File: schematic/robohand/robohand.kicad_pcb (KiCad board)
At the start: 2 copper layers, 1 part, among them U1 ESP32-CAM

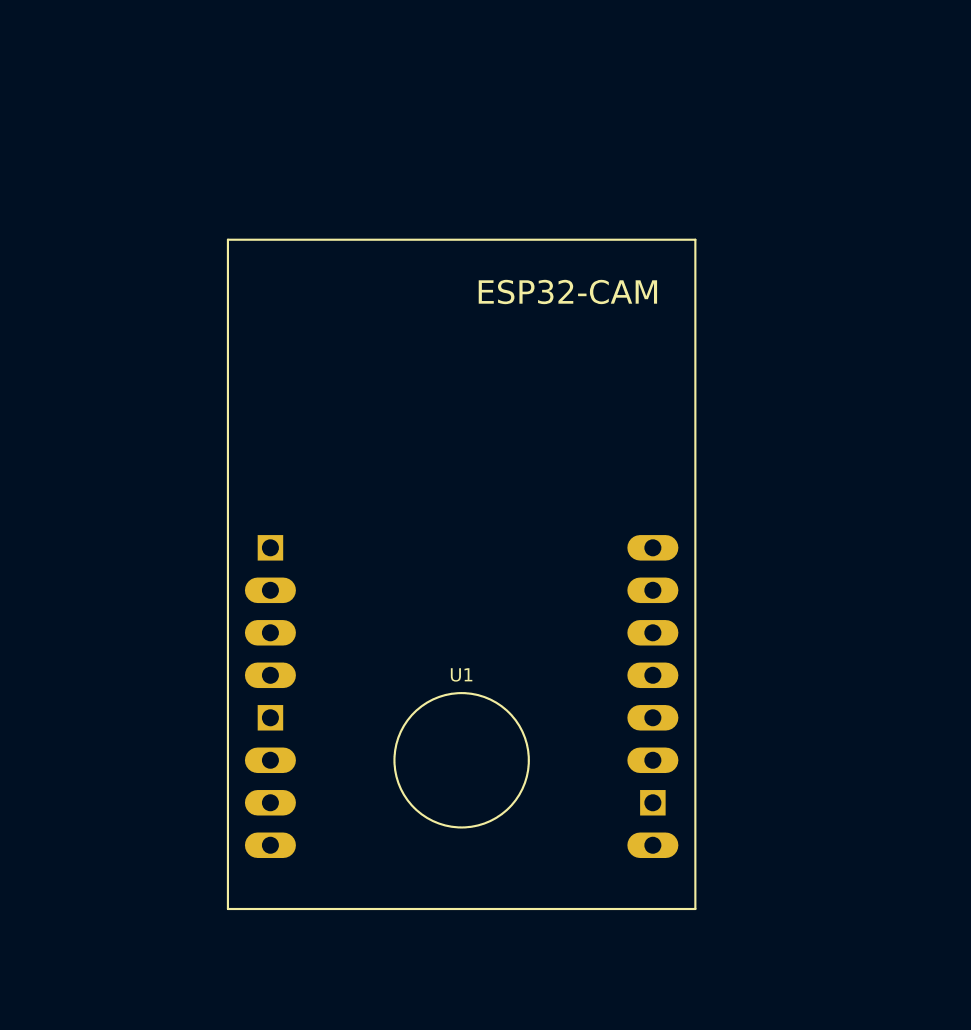
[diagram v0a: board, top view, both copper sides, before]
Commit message: july 2nd
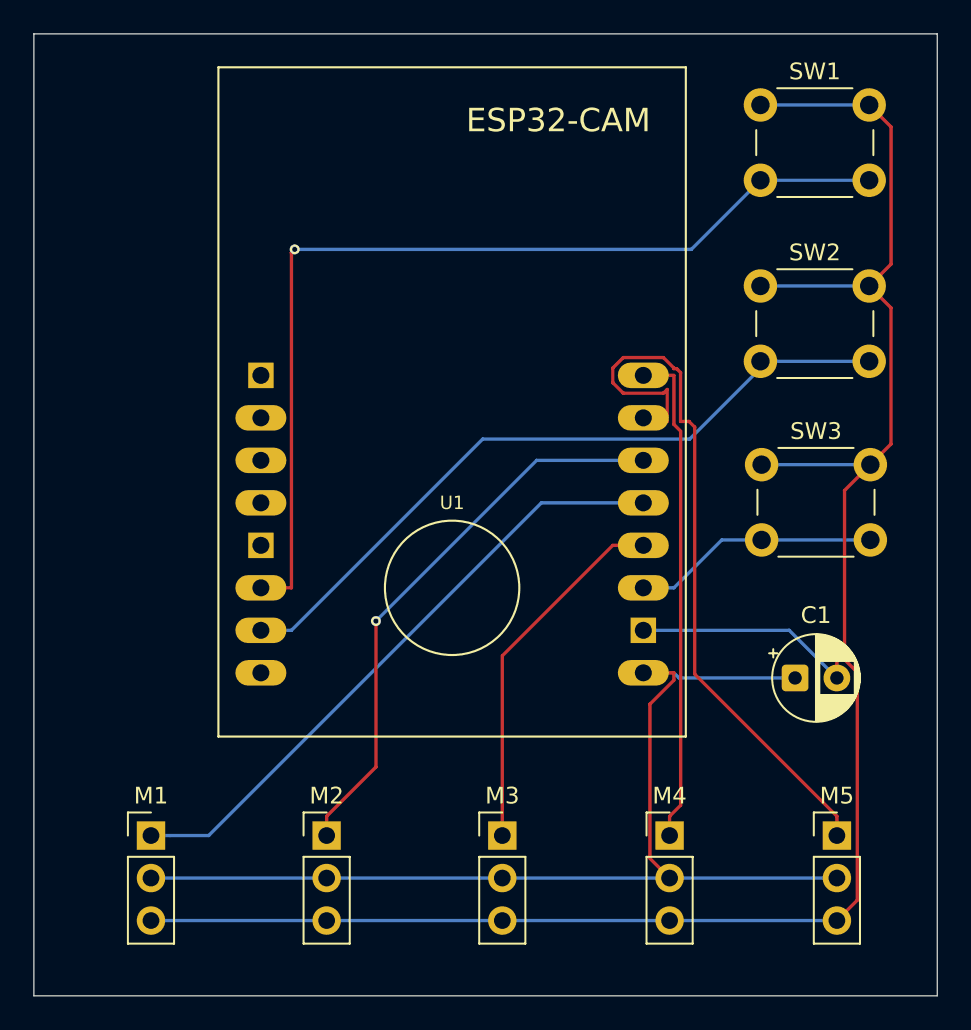
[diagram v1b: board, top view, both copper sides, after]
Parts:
- added C1: C_Polarized, Capacitor_THT:CP_Radial_D5.0mm_P2.50mm, F.Cu at (169.0, 105.5)
- added G***: LOGO, LOGO, B.Cu at (129.5, 77.5)
- added M1: Motor_Servo, Connector_PinHeader_2.54mm:PinHeader_1x03_P2.54mm_Vertical, F.Cu at (130.5, 114.9)
- added M2: Motor_Servo, Connector_PinHeader_2.54mm:PinHeader_1x03_P2.54mm_Vertical, F.Cu at (141.0, 114.9)
- added M3: Motor_Servo, Connector_PinHeader_2.54mm:PinHeader_1x03_P2.54mm_Vertical, F.Cu at (151.5, 114.9)
- added M4: Motor_Servo, Connector_PinHeader_2.54mm:PinHeader_1x03_P2.54mm_Vertical, F.Cu at (161.5, 114.9)
- added M5: Motor_Servo, Connector_PinHeader_2.54mm:PinHeader_1x03_P2.54mm_Vertical, F.Cu at (171.5, 114.9)
- added SW1: SW_SPST, Button_Switch_THT:SW_PUSH_6mm_H5mm, F.Cu at (166.9, 71.2)
- added SW2: SW_SPST, Button_Switch_THT:SW_PUSH_6mm_H5mm, F.Cu at (166.9, 82.1)
- added SW3: SW_SPST, Button_Switch_THT:SW_PUSH_6mm_H5mm, F.Cu at (167.0, 92.8)
- moved U1 10.3 mm to (148.5, 95.0)
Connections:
- U1 pad P$11: unconnected-(U1-GPIO12-PadP$11) -> Net-(SW3-B)
- U1 pad P$12: unconnected-(U1-GPIO13-PadP$12) -> Net-(M3-PWM)
- U1 pad P$16: unconnected-(U1-GPIO4-PadP$16) -> Net-(M4-PWM)
- U1 pad P$2: Net-(M5-PWM) (its old number) -> unconnected-(U1-GPIO1-PadP$2)
- U1 pad P$4: Net-(M4-PWM) -> unconnected-(U1-3V3/5V-PadP$4)
- U1 pad P$6: unconnected-(U1-GPIO0-PadP$6) -> Net-(SW1-B)
- U1 pad P$7: unconnected-(U1-GPIO16-PadP$7) -> Net-(SW2-B)
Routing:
- net GND: track 0.00 -> 127.2 mm
- net +5V: track 0.00 -> 65.4 mm
- net Net-(SW1-B): track 0.00 -> 59.3 mm, vias 0 -> 1
- net Net-(M5-PWM): track 0.00 -> 44.4 mm
- net Net-(SW2-B): track 0.00 -> 43.3 mm
- net Net-(M1-PWM): track 0.00 -> 37.7 mm
- net Net-(M2-PWM): track 0.00 -> 34.2 mm, vias 0 -> 1
- net Net-(M4-PWM): track 0.00 -> 29.8 mm
- net Net-(M3-PWM): track 0.00 -> 21.9 mm
- net Net-(SW3-B): track 0.00 -> 14.8 mm
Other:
- board outline added: 54 x 57.5 mm
